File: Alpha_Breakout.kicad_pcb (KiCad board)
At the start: 4 copper layers, 66.7 x 74.4 mm, 160 parts, among them IC1 LM66200DRLR, J10 Conn_01x03, J11 Conn_01x03, J12 Conn_01x03, J14 Conn_01x03, J15 Conn_01x03, J16 Conn_01x03, J18 Conn_01x02, J19 Conn_01x02, J2 USB_C_Receptacle_USB2.0_16P, J20 Conn_01x02, J21 Conn_01x02, J22 Conn_01x02, J23 Conn_01x02, J24 Conn_01x04, J25 Conn_01x02, J26 Conn_01x02, J27 Conn_01x02, J28 Conn_01x02, J29 Conn_01x02, J3 Conn_01x03, J30 Conn_01x04, J31 Conn_01x02, J33 Conn_01x02, J34 Conn_01x02, J35 Conn_02x06_Odd_Even, J36 Conn_01x02, J4 Conn_01x03, J5 Conn_01x03, J7 Conn_01x03, J8 Conn_01x03, J9 Conn_01x03, Q1 CSD13381F4, Q2 CSD13381F4, Q3 CSD13381F4, Q4 CSD13381F4, Q5 SSM3J328R, Q6 L2N7002SLLT1G, SW1 SW_Push, SW2 SW_Push, U1 STM32F103C8Tx, U10 LP2985-3.3, U11 SP3485EN, U12 ADS1231ID, U13 TCA9517ADGK, U2 CH340N, U3 ADS7828, U4 ADS7828, U5 MAX31856, U6 MAX31856, U7 MAX31856, U8 MAX31856, U9 AP63203WU

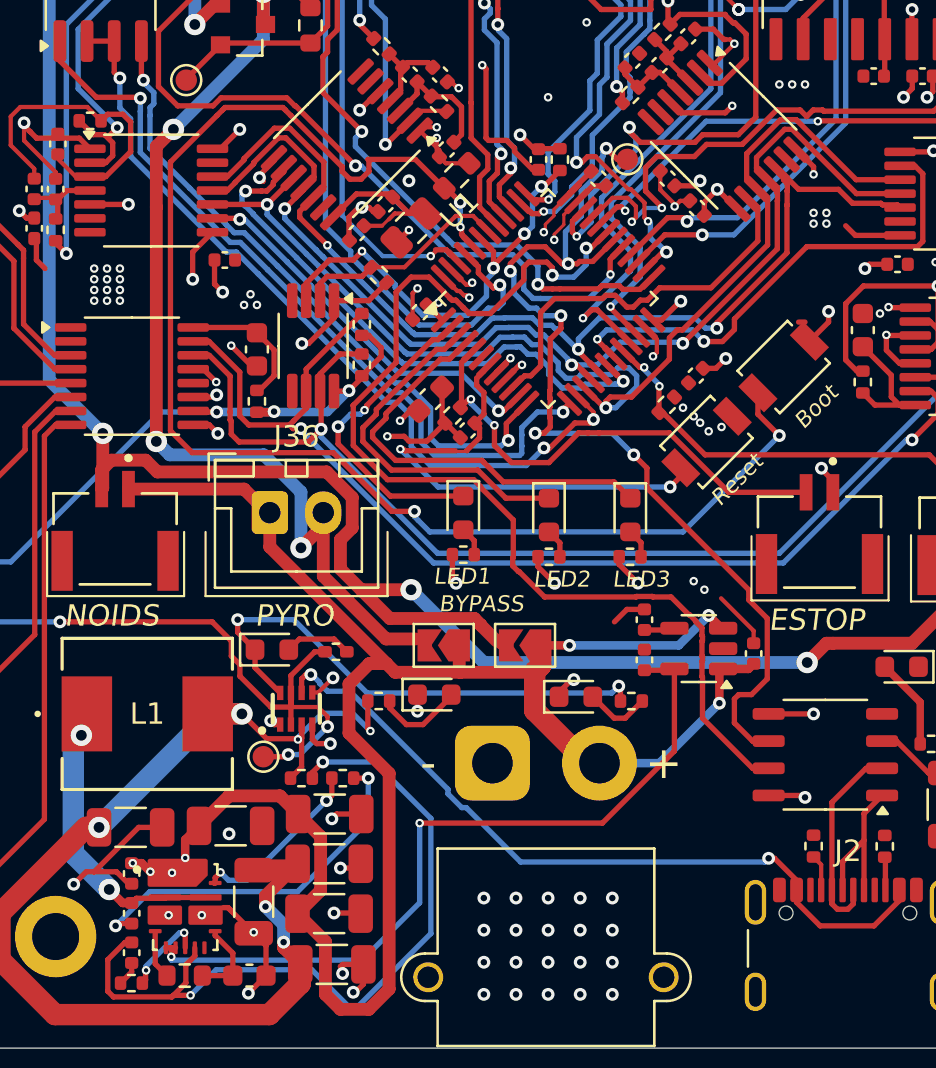
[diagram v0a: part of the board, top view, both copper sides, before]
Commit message: fixed warnings⚠️
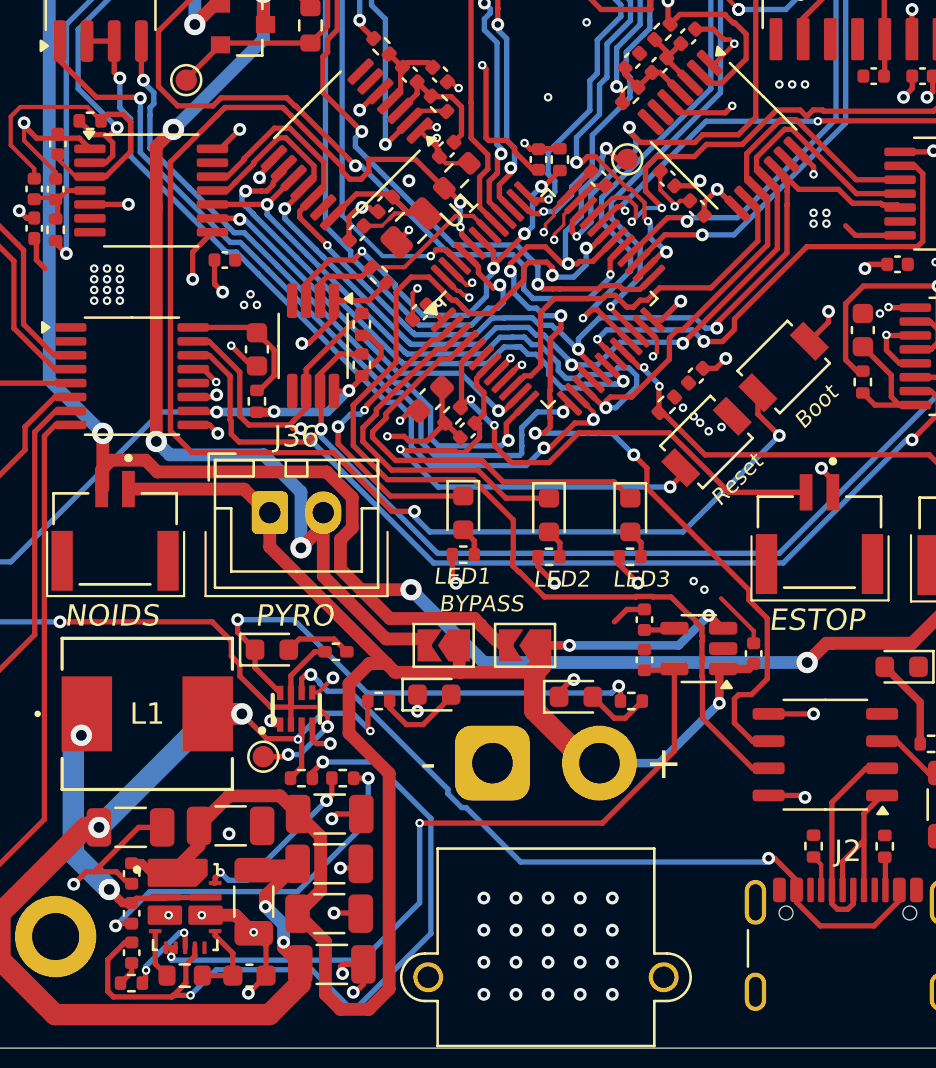
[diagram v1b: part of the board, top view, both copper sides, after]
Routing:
- net +BATT: track 91.5 -> 92.5 mm, vias 7 -> 3
- net GND: track 112.2 -> 112.7 mm
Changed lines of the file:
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@@
 	)
 	(segment
-		(start 134.65 131.348)
-		(end 133.451 130.149)
-		(width 0.25)
-		(layer "F.Cu")
-		(net 5)
-	)
-	(segment
 		(start 141.90707 97.728249)
 		(end 141.13941 96.960589)
@@
 	)
 	(segment
+		(start 132.225 130.5005)
+		(end 133.8025 130.5005)
+		(width 0.6)
+		(layer "F.Cu")
+		(net 5)
+	)
+	(segment
 		(start 145.614222 94.314222)
 		(end 145.5 94.2)
@@
 	)
 	(segment
-		(start 133.451 130.149)
-		(end 133.222166 130.149)
-		(width 0.25)
-		(layer "F.Cu")
-		(net 5)
-	)
-	(segment
 		(start 144.224019 91.875981)
 		(end 144.224019 91.871106)
@@
 	)
 	(segment
-		(start 133.652 130.35)
-		(end 133.451 130.149)
-		(width 0.25)
-		(layer "F.Cu")
-		(net 5)
-	)
-	(segment
 		(start 139.3 134.2)
 		(end 139.3 134.1)
@@
 	)
 	(segment
+		(start 133.8025 130.5005)
+		(end 134.65 131.348)
+		(width 0.6)
+		(layer "F.Cu")
+		(net 5)
+	)
+	(segment
 		(start 123.925 93.625)
 		(end 123.925 93.491942)
@@
 	)
 	(segment
+		(start 132.095 126.33)
+		(end 132.095 127.263)
+		(width 0.6)
+		(layer "F.Cu")
+		(net 7)
+	)
+	(segment
 		(start 149.4 117.9)
 		(end 148.049998 117.9)
@@
 	)
 	(segment
+		(start 132.095 127.263)
+		(end 130.835 128.523)
+		(width 0.6)
+		(layer "F.Cu")
+		(net 7)
+	)
+	(segment
 		(start 157.760002 118.999998)
 		(end 158 118.76)
@@
 	)
 	(segment
-		(start 131.45 127.793768)
-		(end 131.45 127.829123)
-		(width 0.35)
-		(layer "F.Cu")
-		(net 7)
-	)
-	(segment
 		(start 156.4 119.174998)
 		(end 156.575 118.999998)
@@
 	)
 	(segment
-		(start 131.45 126.975)
-		(end 131.45 127.793768)
-		(width 0.4)
-		(layer "F.Cu")
-		(net 7)
-	)
-	(segment
 		(start 134.2 110.6)
 		(end 128.8 110.6)
@@
 	)
 	(segment
-		(start 132.095 126.33)
-		(end 131.45 126.975)
-		(width 0.4)
-		(layer "F.Cu")
-		(net 7)
-	)
-	(segment
 		(start 135.4 111.7)
 		(end 135.3 111.7)
@@
 	)
 	(via
-		(at 130.835 128.523)
-		(size 0.4)
-		(drill 0.2)
-		(layers "F.Cu" "B.Cu")
-		(net 7)
-	)
-	(via
 		(at 155.9 116.5)
 		(size 0.6)
@@
 	)
 	(via
-		(at 129.820768 128.473)
-		(size 0.4)
-		(drill 0.2)
-		(layers "F.Cu" "B.Cu")
-		(net 7)
-	)
-	(via
-		(at 129 128.073)
-		(size 0.4)
-		(drill 0.2)
-		(layers "F.Cu" "B.Cu")
-		(net 7)
-	)
-	(via
 		(at 156.4 120.6)
 		(size 0.6)
@@
 		(net 7)
 	)
-	(via
-		(at 131.45 127.829123)
-		(size 0.4)
-		(drill 0.2)
-		(layers "F.Cu" "B.Cu")
-		(net 7)
-	)
 	(segment
 		(start 154.5 117.9)
@@
 	)
 	(segment
-		(start 160.1 102.8)
-		(end 160.4 102.8)
-		(width 0.25)
-		(layer "F.Cu")
-		(net 9)
-	)
-	(segment
 		(start 144.268633 101.348827)
 		(end 144.159739 101.348827)
@@
 	)
 	(segment
-		(start 147.760049 94.725)
-		(end 147.091281 94.056232)
-		(width 0.25)
-		(layer "F.Cu")
-		(net 9)
-	)
-	(segment
 		(start 154.4 102)
 		(end 154.6 101.8)
@@
 	)
 	(segment
-		(start 147.95 94.725)
-		(end 147.760049 94.725)
-		(width 0.25)
-		(layer "F.Cu")
-		(net 9)
-	)
-	(segment
 		(start 165.392868 89.587132)
 		(end 165.392868 88.207132)
@@
 	)
 	(segment
+		(start 147.584074 94.725)
+		(end 147.297975 94.438901)
+		(width 0.25)
+		(layer "F.Cu")
+		(net 9)
+	)
+	(segment
 		(start 166.35 94.85)
 		(end 166.4 94.8)
@@
 	)
 	(segment
+		(start 147.95 94.725)
+		(end 147.584074 94.725)
+		(width 0.25)
+		(layer "F.Cu")
+		(net 9)
+	)
+	(segment
 		(start 161.7 110.2)
 		(end 161.1 109.6)
@@
 	)
 	(segment
+		(start 147.760049 94.725)
+		(end 147.95 94.725)
+		(width 0.25)
+		(layer "F.Cu")
+		(net 9)
+	)
+	(segment
 		(start 140.021248 101.8)
 		(end 138.4 101.8)
@@
 	)
 	(via
-		(at 147.091281 94.056232)
-		(size 0.6)
-		(drill 0.3)
-		(layers "F.Cu" "B.Cu")
-		(net 9)
-	)
-	(via
 		(at 143.286681 101.891398)
 		(size 0.4)
@@
 	)
 	(via
+		(at 147.297975 94.438901)
+		(size 0.4)
+		(drill 0.2)
+		(layers "F.Cu" "B.Cu")
+		(net 9)
+	)
+	(via
 		(at 156.3 96.6)
 		(size 0.6)
@@
 		(min_thickness 0.25)
 		(filled_areas_thickness no)
-		(fill
+		(fill yes
 			(thermal_gap 0.5)
 			(thermal_bridge_width 0.5)
@@
 		(min_thickness 0.25)
 		(filled_areas_thickness no)
-		(fill
+		(fill yes
 			(thermal_gap 0.5)
 			(thermal_bridge_width 0.5)
@@
 		(min_thickness 0.25)
 		(filled_areas_thickness no)
-		(fill
+		(fill yes
 			(thermal_gap 0.5)
 			(thermal_bridge_width 0.5)
@@
 		(min_thickness 0.25)
 		(filled_areas_thickness no)
-		(fill
+		(fill yes
 			(thermal_gap 0.5)
 			(thermal_bridge_width 0.5)
@@
 		(min_thickness 0.25)
 		(filled_areas_thickness no)
-		(fill
+		(fill yes
 			(thermal_gap 0.5)
 			(thermal_bridge_width 0.5)
@@
 		(min_thickness 0.25)
 		(filled_areas_thickness no)
-		(fill
+		(fill yes
 			(thermal_gap 0.5)
 			(thermal_bridge_width 0.5)
